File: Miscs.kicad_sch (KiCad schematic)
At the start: 14 parts, among them U7 THGBMUG6C1LBAIL

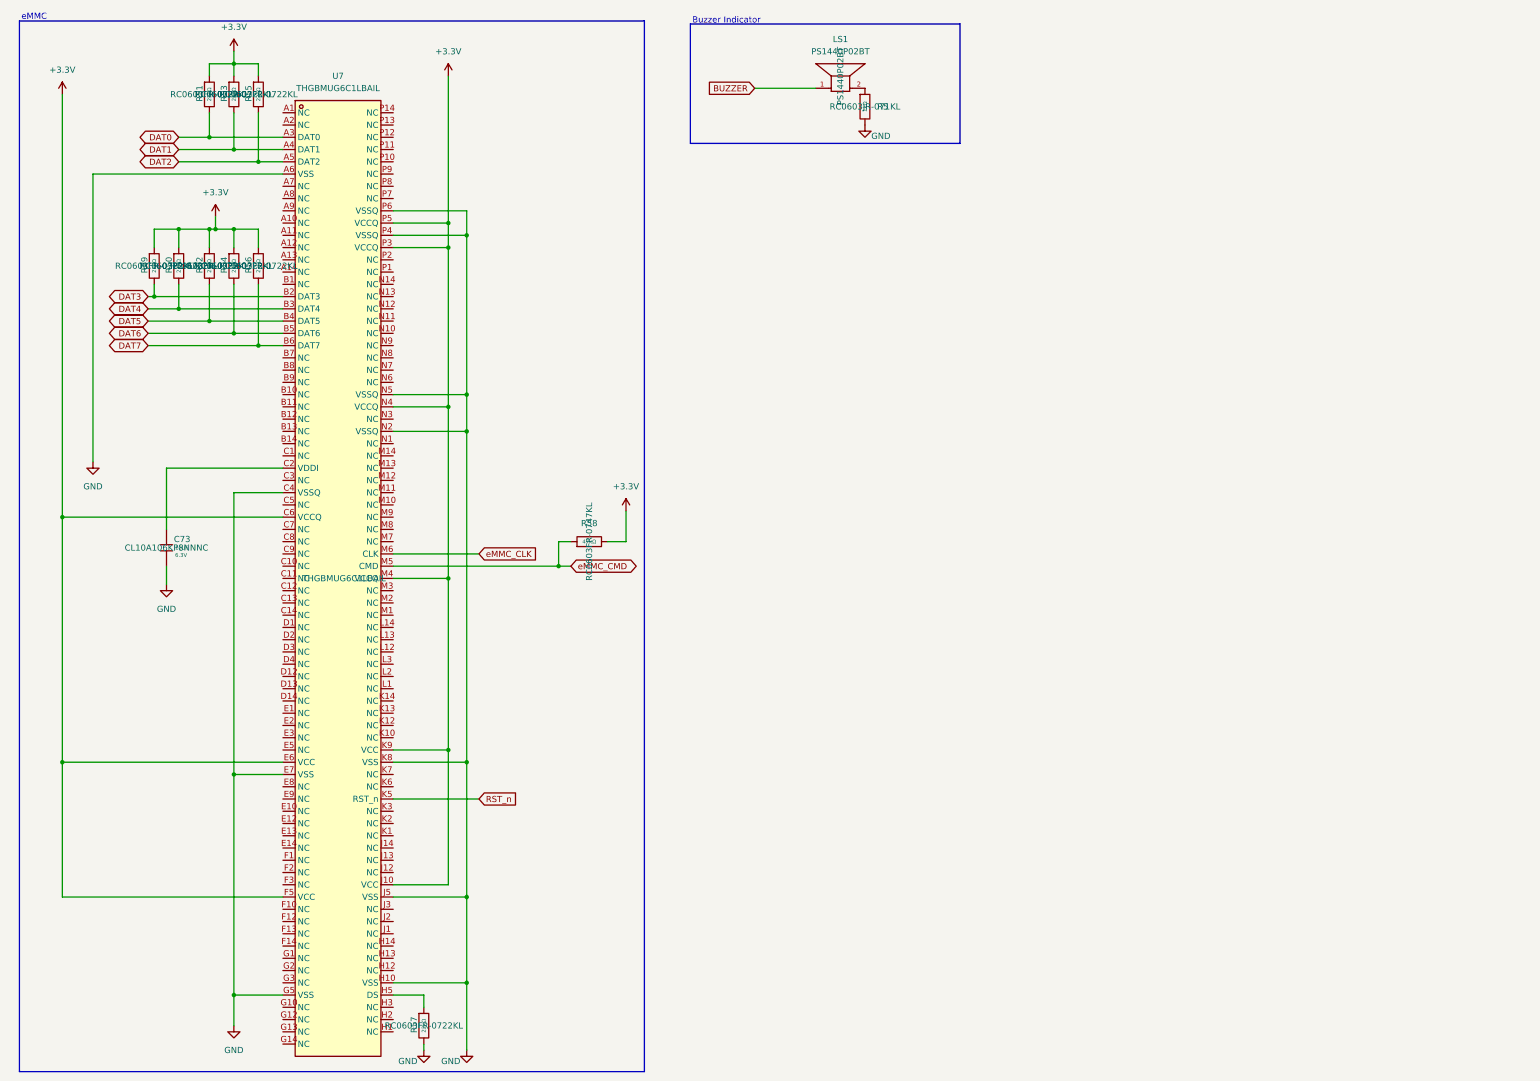
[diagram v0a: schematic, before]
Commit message: Complete Redesign
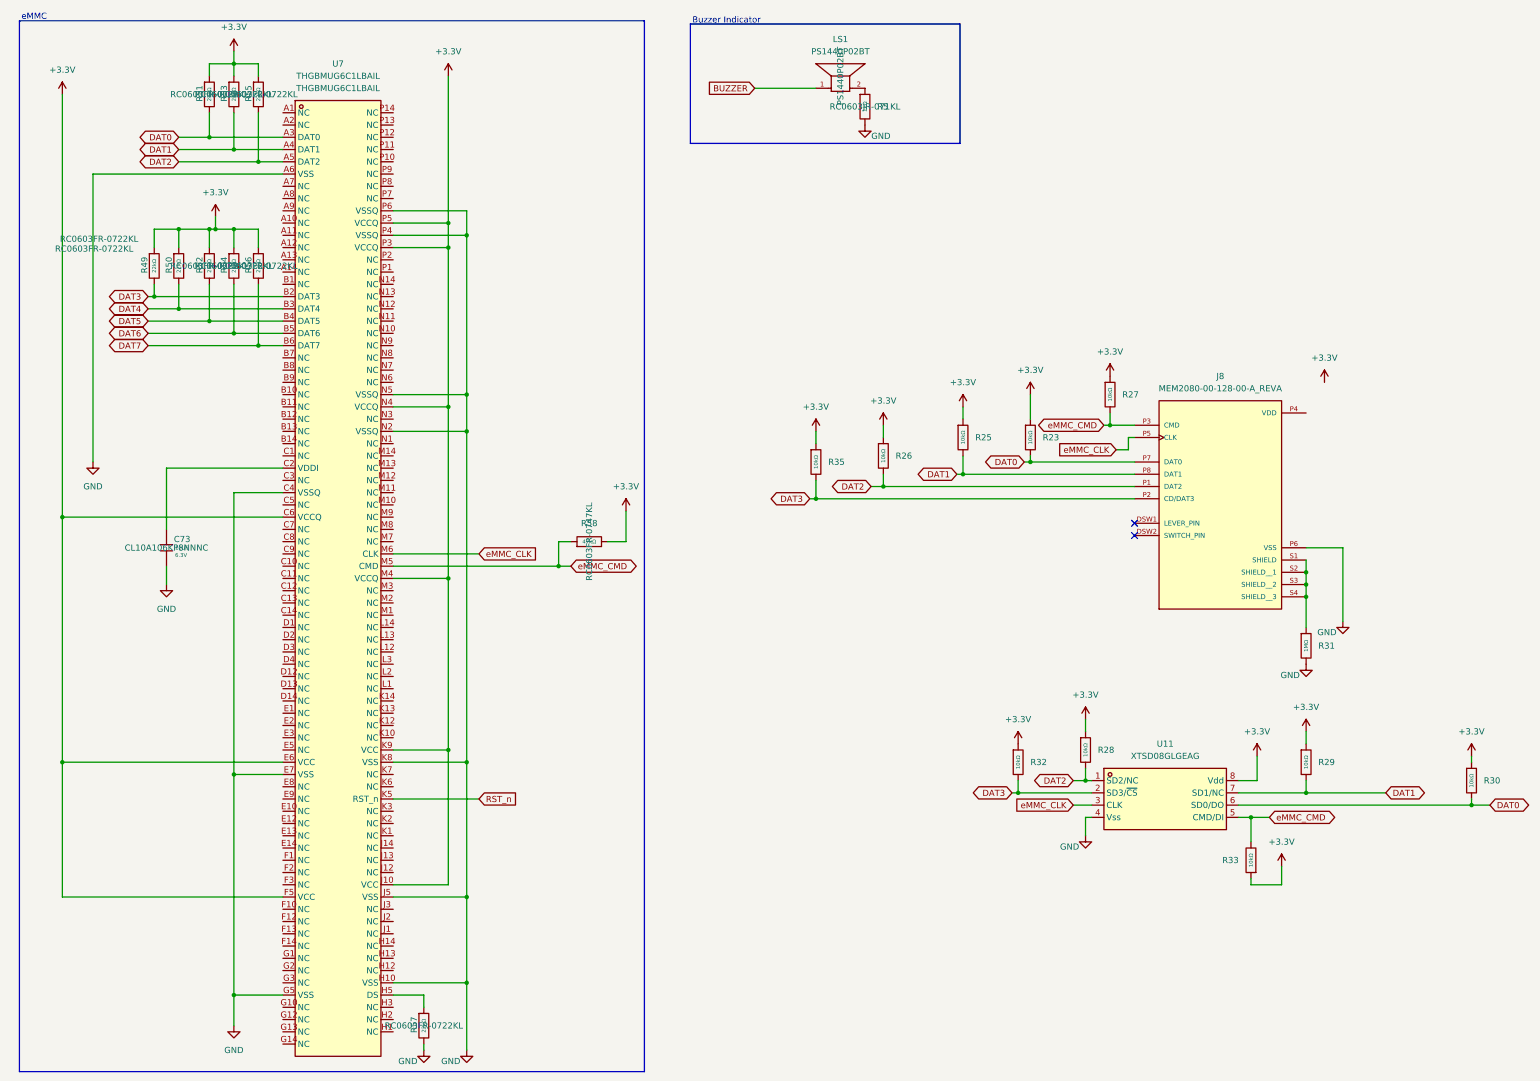
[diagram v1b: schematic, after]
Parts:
- added J8: MEM2080-00-128-00-A_REVA, SDCard:GCT_MEM2080-00-128-00-A_REVA, symbol MEM2080-00-128-00-A_REVA:MEM2080-00-128-00-A_REVA
- added R23, R25, R26, R27, R28, R29, R30, R32, R33, R35: 10kΩ, PCM_JLCPCB:R_0603, symbol PCM_JLCPCB-Resistors:0603,10kΩ
- added R31: 1MΩ, PCM_JLCPCB:R_0603, symbol PCM_JLCPCB-Resistors:0603,1MΩ
- added U11: XTSD08GLGEAG, EasyEDA:LGA-8_L6.0-W8.0-P1.27-BL, symbol EasyEDA:XTSD08GLGEAG
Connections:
- net +3.3V: now also R23.1, R25.1, R26.1, R27.1, R28.1, R29.1, R30.1, R32.1, R33.1, R35.1, U11.8 (Vdd)
- net DAT0: now also J8.P7 (DAT0), R23.2, R30.2, U11.6 (SD0/DO)
- net DAT1: now also J8.P8 (DAT1), R25.2, R29.2, U11.7 (SD1/NC)
- net DAT2: now also J8.P1 (DAT2), R26.2, R28.2, U11.1 (SD2/NC)
- net DAT3: now also J8.P2 (CD/DAT3), R32.2, R35.2, U11.2 (SD3/~{CS})
- net GND: now also J8.P6 (VSS), R31.2, U11.4 (Vss)
- net eMMC_CLK: now also J8.P5 (CLK), U11.3 (CLK)
- net eMMC_CMD: now also J8.P3 (CMD), R27.2, R33.2, U11.5 (CMD/DI)
- new net: J8.S1 (SHIELD), J8.S2 (SHIELD__1), J8.S3 (SHIELD__2), J8.S4 (SHIELD__3), R31.1
- no-connect marks 0 -> 2

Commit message: 1
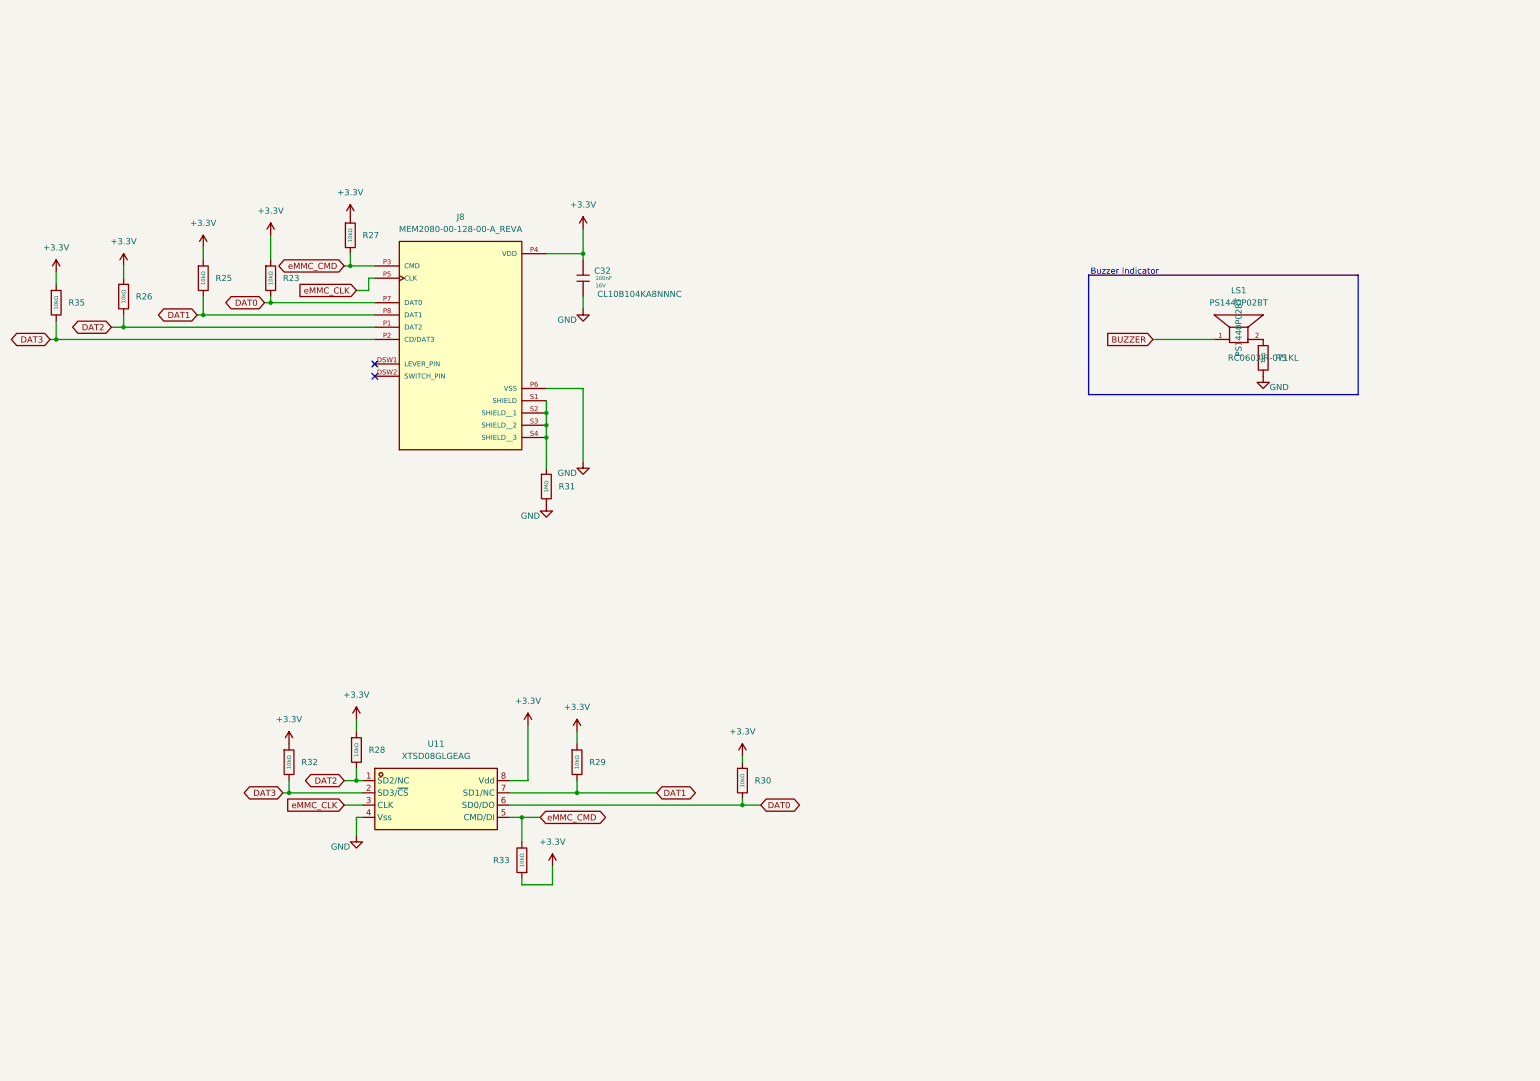
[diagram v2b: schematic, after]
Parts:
- removed C73: 10uF, PCM_JLCPCB:C_0603, symbol PCM_JLCPCB-Capacitors:0402,10uF
- removed R49, R50, R51, R52, R53, R54, R55, R56, R57: 22kΩ, PCM_JLCPCB:R_0603, symbol PCM_JLCPCB-Resistors:0402,22kΩ
- removed R58: 47kΩ, PCM_JLCPCB:R_0603, symbol PCM_JLCPCB-Resistors:0402,47kΩ
- removed U7: THGBMUG6C1LBAIL, EasyEDA:BGA-153_L13.0-W11.5-P0.50-TL_KLM8G1GEME-B041, symbol EasyEDA:THGBMUG6C1LBAIL
- added C32: 100nF, PCM_JLCPCB:C_0603, symbol PCM_JLCPCB-Capacitors:0402,100nF
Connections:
- net +3.3V: now also J8.P4 (VDD), C32.1
- net GND: now also C32.2
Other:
- note removed: "eMMC"
- moved on the sheet: J8, LS1, R23, R25, R26, R27, R28, R29, R30, R31, R32, R33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
